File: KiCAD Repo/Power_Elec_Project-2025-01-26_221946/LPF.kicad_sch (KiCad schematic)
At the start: 2 parts, among them U1 LM358

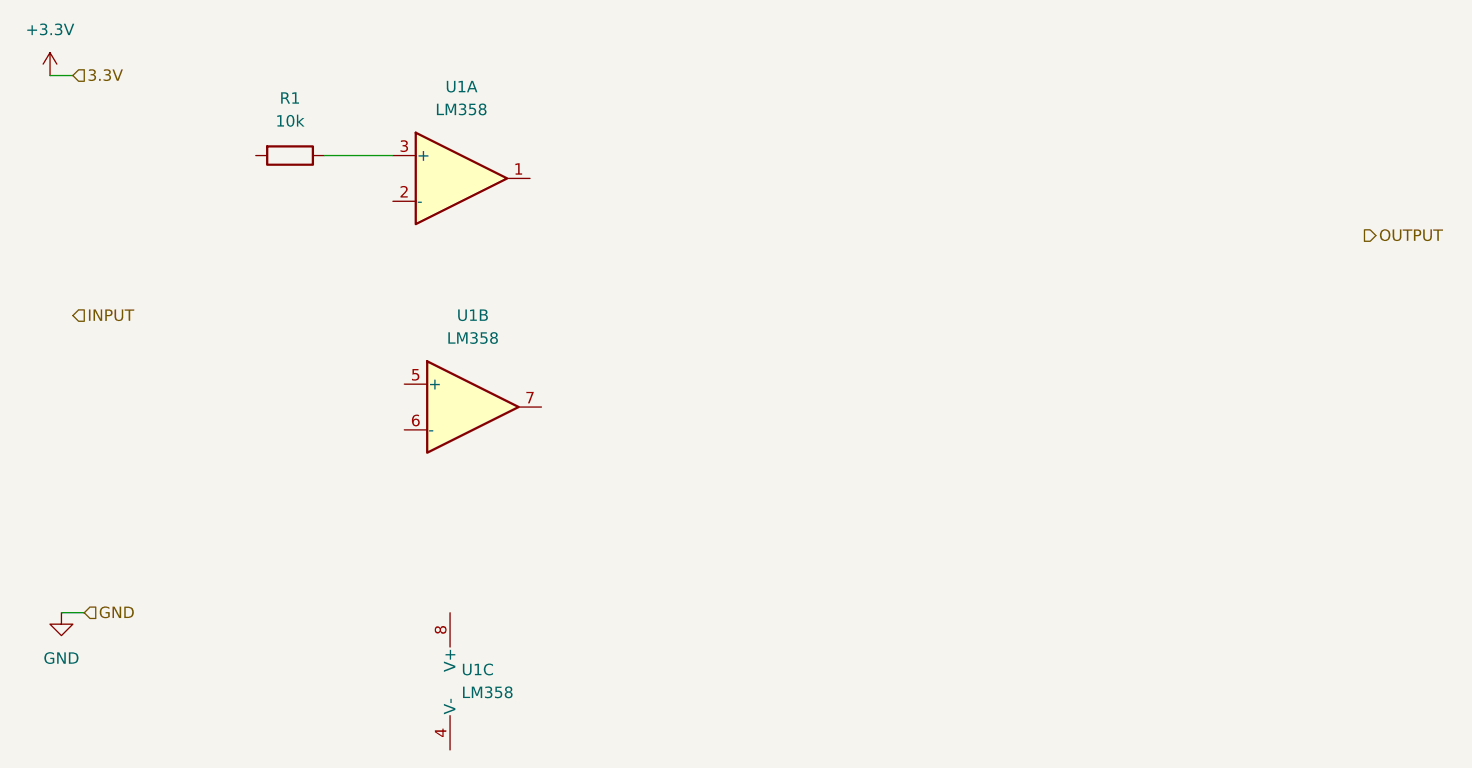
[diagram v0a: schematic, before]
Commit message: lpf
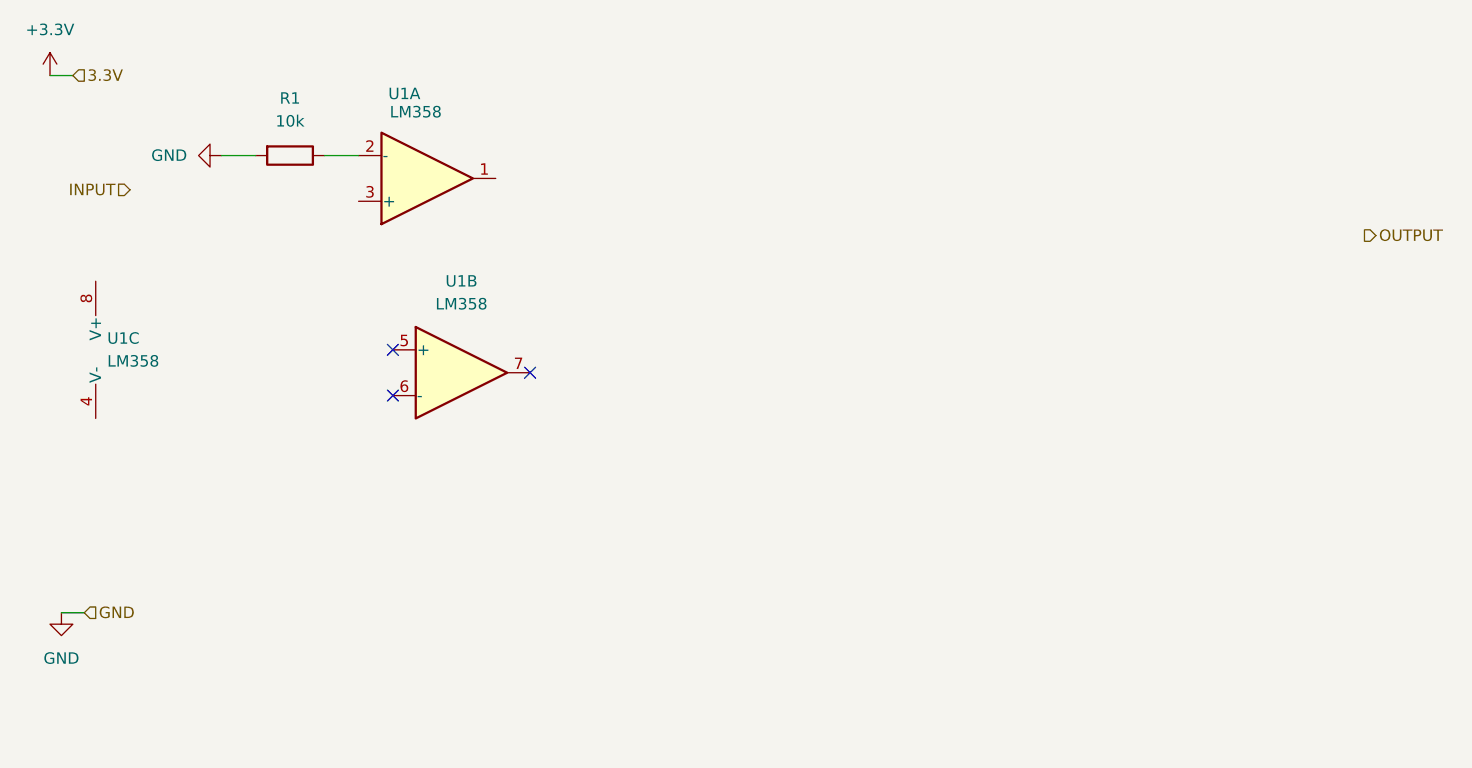
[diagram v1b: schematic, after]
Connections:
- net GND: now also R1.2
- net at R1.1: now also U1.2 (-); no longer U1.3 (+)
- no-connect marks 0 -> 3
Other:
- moved on the sheet: U1A, U1B, U1C
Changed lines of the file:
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@@
 	(generator_version "8.0")
 	(paper "A4")
+	(no_connect
+		(at 69.85 72.39)
+	)
+	(no_connect
+		(at 69.85 77.47)
+	)
+	(no_connect
+		(at 85.09 74.93)
+	)
+	(wire
+		(pts
+			(xy 50.8 50.8) (xy 54.61 50.8)
+		)
+		(stroke
+			(width 0)
+			(type default)
+		)
+	)
+	(wire
+		(pts
+			(xy 62.23 50.8) (xy 66.04 50.8)
+		)
+		(stroke
+			(width 0)
+			(type default)
+		)
+	)
 	(wire
 		(pts
 			(xy 31.75 41.91) (xy 34.29 41.91)
-		)
-		(stroke
-			(width 0)
-			(type default)
-		)
-	)
-	(wire
-		(pts
-			(xy 62.23 50.8) (xy 69.85 50.8)
 		)
 		(stroke
@@
 	(hierarchical_label "INPUT"
 		(shape input)
-		(at 34.29 68.58 0)
+		(at 40.64 54.61 180)
 		(effects
 			(font
 				(size 1.27 1.27)
 			)
-			(justify left)
+			(justify right)
 		)
 	)
@@
 	(symbol
 		(lib_id "Amplifier_Operational:LM358")
-		(at 78.74 109.22 0)
+		(at 39.37 72.39 0)
 		(unit 3)
 		(exclude_from_sim no)
@@
 		(fields_autoplaced yes)
 		(property "Reference" "U1"
-			(at 77.47 107.9499 0)
+			(at 38.1 71.1199 0)
 			(effects
 				(font
@@
 		)
 		(property "Value" "LM358"
-			(at 77.47 110.4899 0)
+			(at 38.1 73.6599 0)
 			(effects
 				(font
@@
 		)
 		(property "Footprint" "Package_SO:VSSOP-8_3x3mm_P0.65mm"
-			(at 78.74 109.22 0)
+			(at 39.37 72.39 0)
 			(effects
 				(font
@@
 		)
 		(property "Datasheet" "http://www.ti.com/lit/ds/symlink/lm2904-n.pdf"
-			(at 78.74 109.22 0)
+			(at 39.37 72.39 0)
 			(effects
 				(font
@@
 		)
 		(property "Description" "Low-Power, Dual Operational Amplifiers, DIP-8/SOIC-8/TO-99-8"
-			(at 78.74 109.22 0)
+			(at 39.37 72.39 0)
 			(effects
 				(font
@@
 		)
 		(property "Part Number" "LM358DGKR"
-			(at 78.74 109.22 0)
+			(at 39.37 72.39 0)
 			(effects
 				(font
@@
 	(symbol
 		(lib_id "Amplifier_Operational:LM358")
-		(at 78.74 78.74 0)
+		(at 77.47 74.93 0)
 		(unit 2)
 		(exclude_from_sim no)
@@
 		(fields_autoplaced yes)
 		(property "Reference" "U1"
-			(at 78.74 68.58 0)
+			(at 77.47 64.77 0)
 			(effects
 				(font
@@
 		)
 		(property "Value" "LM358"
-			(at 78.74 71.12 0)
+			(at 77.47 67.31 0)
 			(effects
 				(font
@@
 		)
 		(property "Footprint" "Package_SO:VSSOP-8_3x3mm_P0.65mm"
-			(at 78.74 78.74 0)
+			(at 77.47 74.93 0)
 			(effects
 				(font
@@
 		)
 		(property "Datasheet" "http://www.ti.com/lit/ds/symlink/lm2904-n.pdf"
-			(at 78.74 78.74 0)
+			(at 77.47 74.93 0)
 			(effects
 				(font
@@
 		)
 		(property "Description" "Low-Power, Dual Operational Amplifiers, DIP-8/SOIC-8/TO-99-8"
-			(at 78.74 78.74 0)
+			(at 77.47 74.93 0)
 			(effects
 				(font
@@
 		)
 		(property "Part Number" "LM358DGKR"
-			(at 78.74 78.74 0)
+			(at 77.47 74.93 0)
 			(effects
 				(font
@@
 	)
 	(symbol
+		(lib_id "power:GND")
+		(at 50.8 50.8 270)
+		(unit 1)
+		(exclude_from_sim no)
+		(in_bom yes)
+		(on_board yes)
+		(dnp no)
+		(fields_autoplaced yes)
+		(property "Reference" "#PWR011"
+			(at 44.45 50.8 0)
+			(effects
+				(font
+					(size 1.27 1.27)
+				)
+				(hide yes)
+			)
+		)
+		(property "Value" "GND"
+			(at 46.99 50.7999 90)
+			(effects
+				(font
+					(size 1.27 1.27)
+				)
+				(justify right)
+			)
+		)
+		(property "Footprint" ""
+			(at 50.8 50.8 0)
+			(effects
+				(font
+					(size 1.27 1.27)
+				)
+				(hide yes)
+			)
+		)
+		(property "Datasheet" ""
+			(at 50.8 50.8 0)
+			(effects
+				(font
+					(size 1.27 1.27)
+				)
+				(hide yes)
+			)
+		)
+		(property "Description" "Power symbol creates a global label with name \"GND\" , ground"
+			(at 50.8 50.8 0)
+			(effects
+				(font
+					(size 1.27 1.27)
+				)
+				(hide yes)
+			)
+		)
+		(pin "1"
+		)
+		(instances
+			(project "Power_Elec_Project"
+				(path "/ecd51ed2-b30f-41c1-93fa-3d04786e684e/24945a6e-9cf1-4d51-984e-568b86374556"
+					(reference "#PWR011")
+					(unit 1)
+				)
+			)
+		)
+	)
+	(symbol
 		(lib_id "Amplifier_Operational:LM358")
-		(at 77.47 53.34 0)
+		(at 73.66 53.34 0)
+		(mirror x)
 		(unit 1)
 		(exclude_from_sim no)
@@
 		(on_board yes)
 		(dnp no)
-		(fields_autoplaced yes)
 		(property "Reference" "U1"
-			(at 77.47 43.18 0)
+			(at 71.12 43.942 0)
 			(effects
 				(font
@@
 		)
 		(property "Value" "LM358"
-			(at 77.47 45.72 0)
+			(at 72.39 45.974 0)
 			(effects
 				(font
@@
 		)
 		(property "Footprint" "Package_SO:VSSOP-8_3x3mm_P0.65mm"
-			(at 77.47 53.34 0)
+			(at 73.66 53.34 0)
 			(effects
 				(font
@@
 		)
 		(property "Datasheet" "http://www.ti.com/lit/ds/symlink/lm2904-n.pdf"
-			(at 77.47 53.34 0)
+			(at 73.66 53.34 0)
 			(effects
 				(font
@@
 		)
 		(property "Description" "Low-Power, Dual Operational Amplifiers, DIP-8/SOIC-8/TO-99-8"
-			(at 77.47 53.34 0)
+			(at 73.66 53.34 0)
 			(effects
 				(font
@@
 		)
 		(property "Part Number" "LM358DGKR"
-			(at 77.47 53.34 0)
-			(effects
-				(font
+			(at 73.66 53.34 0)
+			(effects
+				(font
